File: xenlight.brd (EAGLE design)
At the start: 160.2 x 80.2 mm, 33 parts, among them IC1 MEGA16-A, IC14 FT232RL, IC2 74HC573D, IC3 74HC573D, IC4 74HC573D, IC5 74HC573D, IC6 74HC573D, IC7 74HC573D, X1 057-010-1, X2 057-010-1, X3 057-010-1, X4 057-010-1, X5 057-010-1, X6 057-010-1, X7 KUSBVX

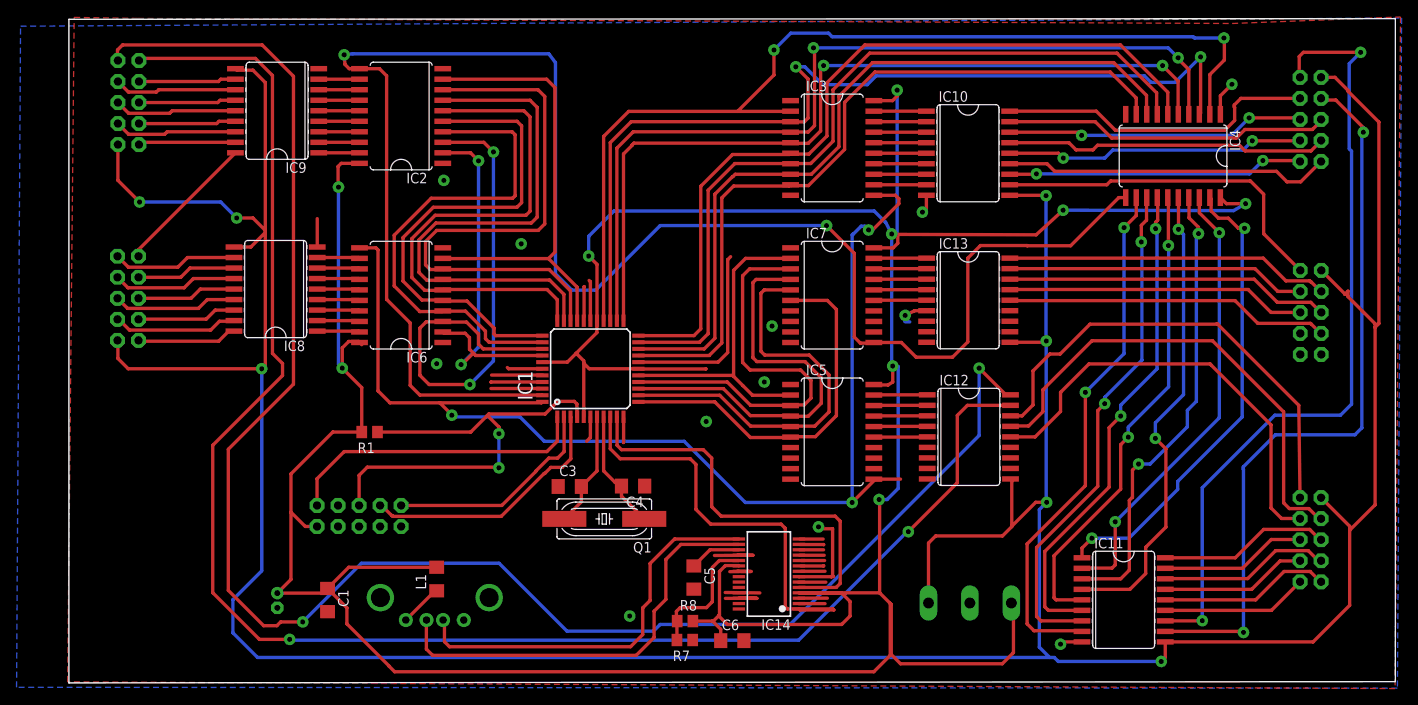
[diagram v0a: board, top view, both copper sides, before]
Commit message: Second version of board, not for homemade production.
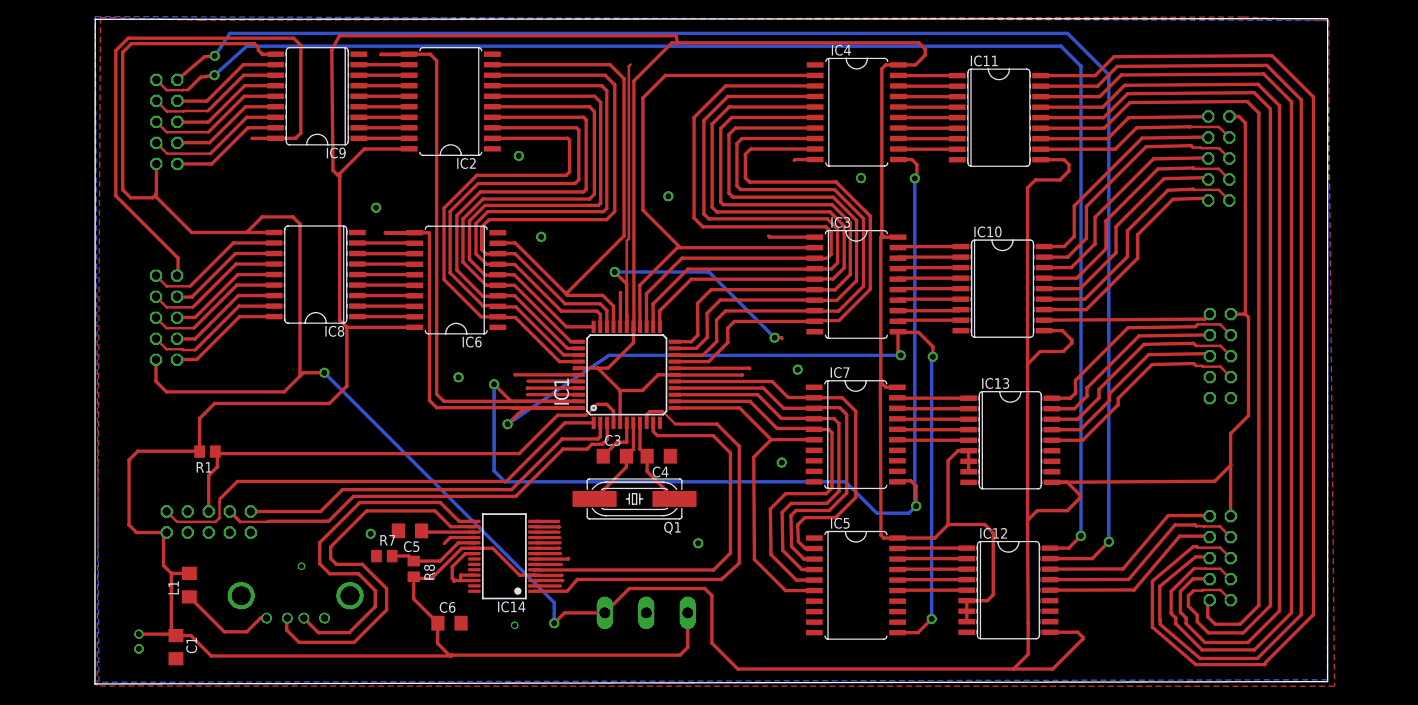
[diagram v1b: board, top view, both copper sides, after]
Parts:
- moved IC11 60.2 mm to (117.9, 68.4)
- moved X9 39.1 mm to (75.3, 8.61)
- moved IC4 38.6 mm to (100.8, 69.1), turned to 270 degrees
- moved R7 37.7 mm to (43.7, 15.5), turned to 0 degrees
- moved C5 34.8 mm to (46.8, 18.5), turned to 180 degrees
- moved C6 34.2 mm to (51.6, 7.37)
- moved R8 33.4 mm to (47.2, 13.9), turned to 270 degrees
- moved IC14 32.0 mm to (58.2, 15.4)
- moved L1 29.9 mm to (20.1, 12.0)
- moved R1 19.7 mm to (22.3, 28.1)
- moved C1 19.2 mm to (18.5, 4.47)
- moved IC12 19.1 mm to (119.1, 11.4)
- moved IC5 18.8 mm to (100.7, 11.9)
- moved X6 18.2 mm to (22.5, 19.6)
- moved IC13 17.7 mm to (119.3, 29.5)
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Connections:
- net GND: no longer IC12.6, IC12.7, IC12.8, IC13.6, IC13.7, IC13.8
- net VCC: now also IC12.6, IC12.7, IC12.8, IC13.6, IC13.7, IC13.8
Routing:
- net N$93: track 20.8 -> 139.3 mm
- net N$94: track 17.7 -> 129.1 mm
- net N$95: track 20.7 -> 124.6 mm
- net N$96: track 17.7 -> 114.2 mm
- net N$97: track 20.8 -> 110.0 mm
- net N$98: track 17.7 -> 97.3 mm
- net N$99: track 96.1 -> 21.3 mm, vias 2 -> 0
- net N$100: track 88.7 -> 24.4 mm, vias 2 -> 0
- net N$55: track 64.0 -> 7.12 mm, vias 2 -> 0
- net N$54: track 61.9 -> 7.12 mm, vias 2 -> 0
- net N$75: track 17.3 -> 70.4 mm
- net N$53: track 59.9 -> 7.12 mm, vias 2 -> 0
- net N$9: track 120.8 -> 69.9 mm, vias 2 -> 0
- net N$52: track 57.6 -> 7.12 mm, vias 2 -> 0
- net N$48: track 57.1 -> 7.12 mm, vias 2 -> 0
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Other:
- board size 160.2 x 80.2 mm -> 148.9 x 80.4 mm
